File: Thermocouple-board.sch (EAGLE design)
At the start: 92 parts, among them J1 RJ45, J10 1X2-3.5MM, J11 1X2-3.5MM, J12 1X2-3.5MM, J13 1X2-3.5MM, J2 RJ45, J3 1981584-1LONGPADS, J4 2.1MMJACKTHM, J5 ST-LINK, J6 HEADER-1X3, J7 UART, SW1 PUSHBUTTON, SW2 PUSHBUTTON, U1 STM32F042K6, U10 MAX31855, U11 MAX31855, U12 MAX31855, U13 MAX31855, U20 EEPROM-I2C, U21 EEPROM-I2C, U30 ST3485, U31 ST3485, U40 LP298XS, U70 TPS25921, Y1 8MHz

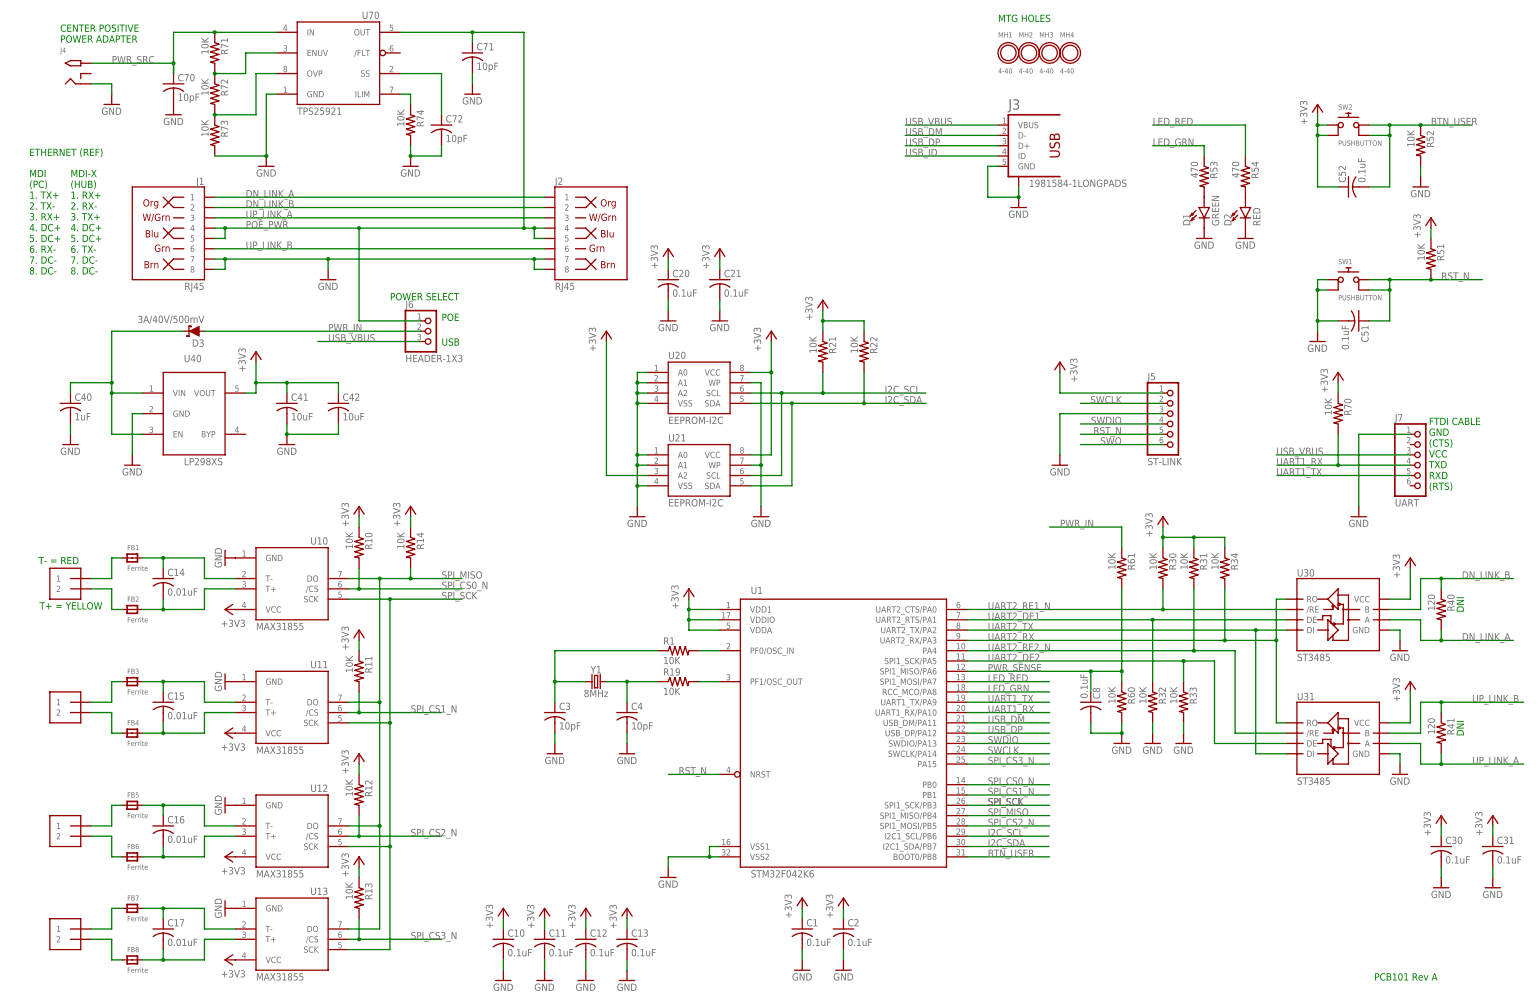
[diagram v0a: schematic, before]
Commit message: Routing complete
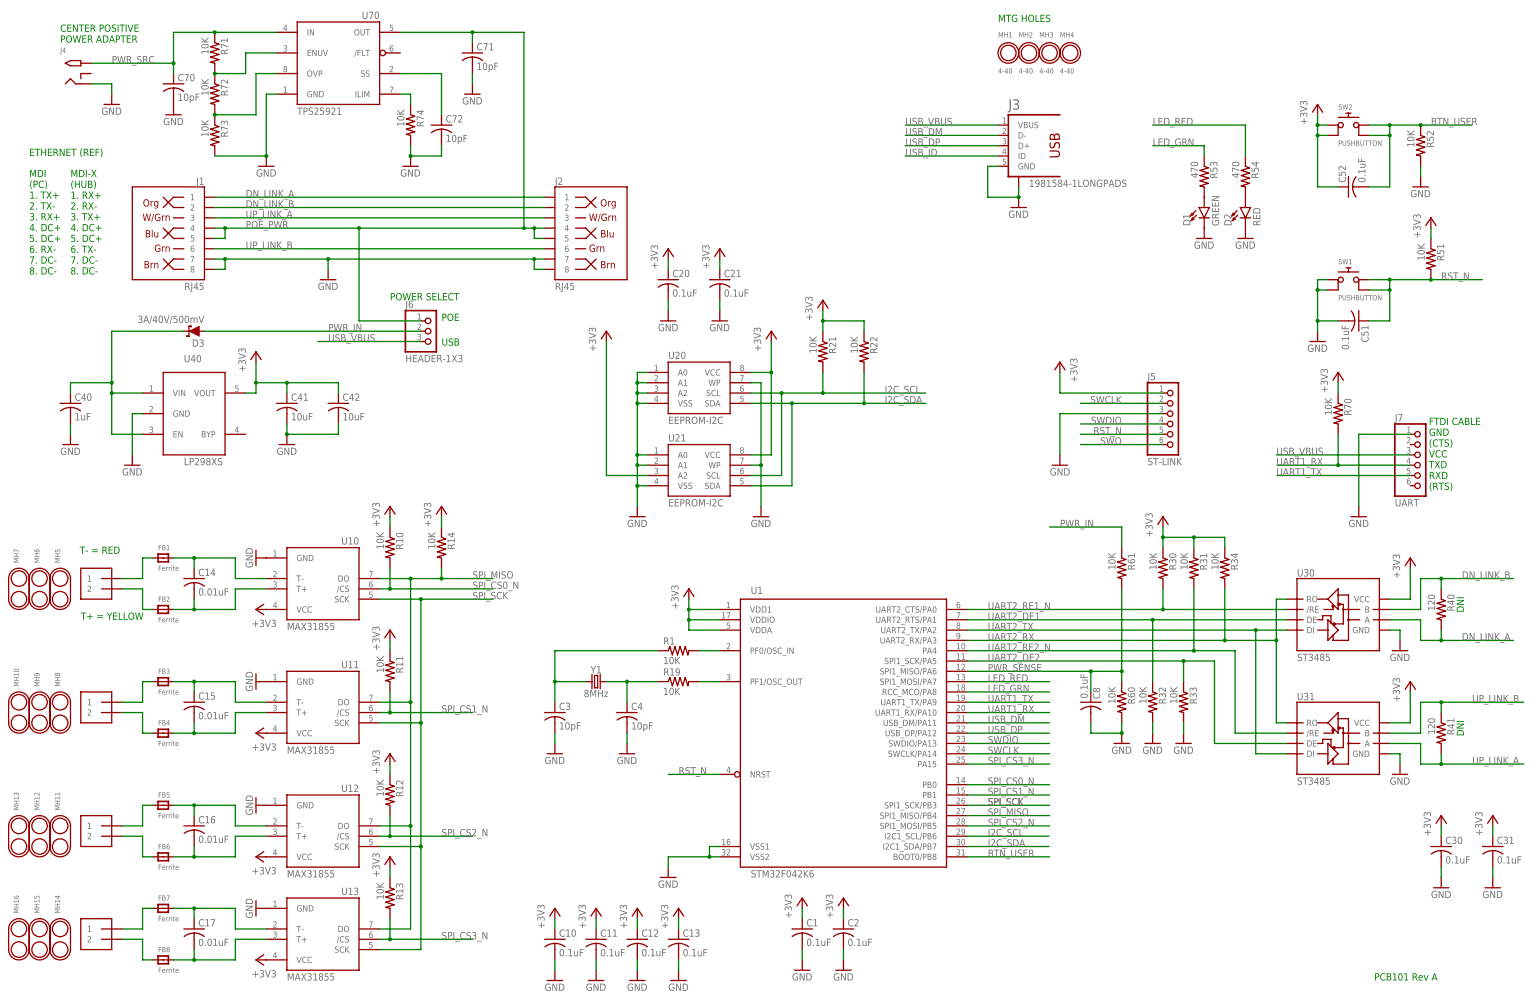
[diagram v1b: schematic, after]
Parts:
- added MH10, MH11, MH12, MH13, MH14, MH15, MH16, MH5, MH6, MH7, MH8, MH9: HOLD_DOWN, Thermocouple-board:HOLD_DOWN
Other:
- moved on the sheet: C10, C11, C12, C13, C14, C15, C16, C17, FB1, FB2, FB3, FB4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
